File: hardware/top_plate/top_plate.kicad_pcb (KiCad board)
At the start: 2 copper layers, 96 x 66 mm, 36 parts, among them J1 Conn_01x04_Male, J2 Conn_01x04, J3 Conn_02x04_Odd_Even, J4 Conn_01x04, Q1 BSS138, Q2 BSS138, SW1 SW_Push, SW2 SW_Push, U1 AP2112K-1.8, U2 ICM-20948

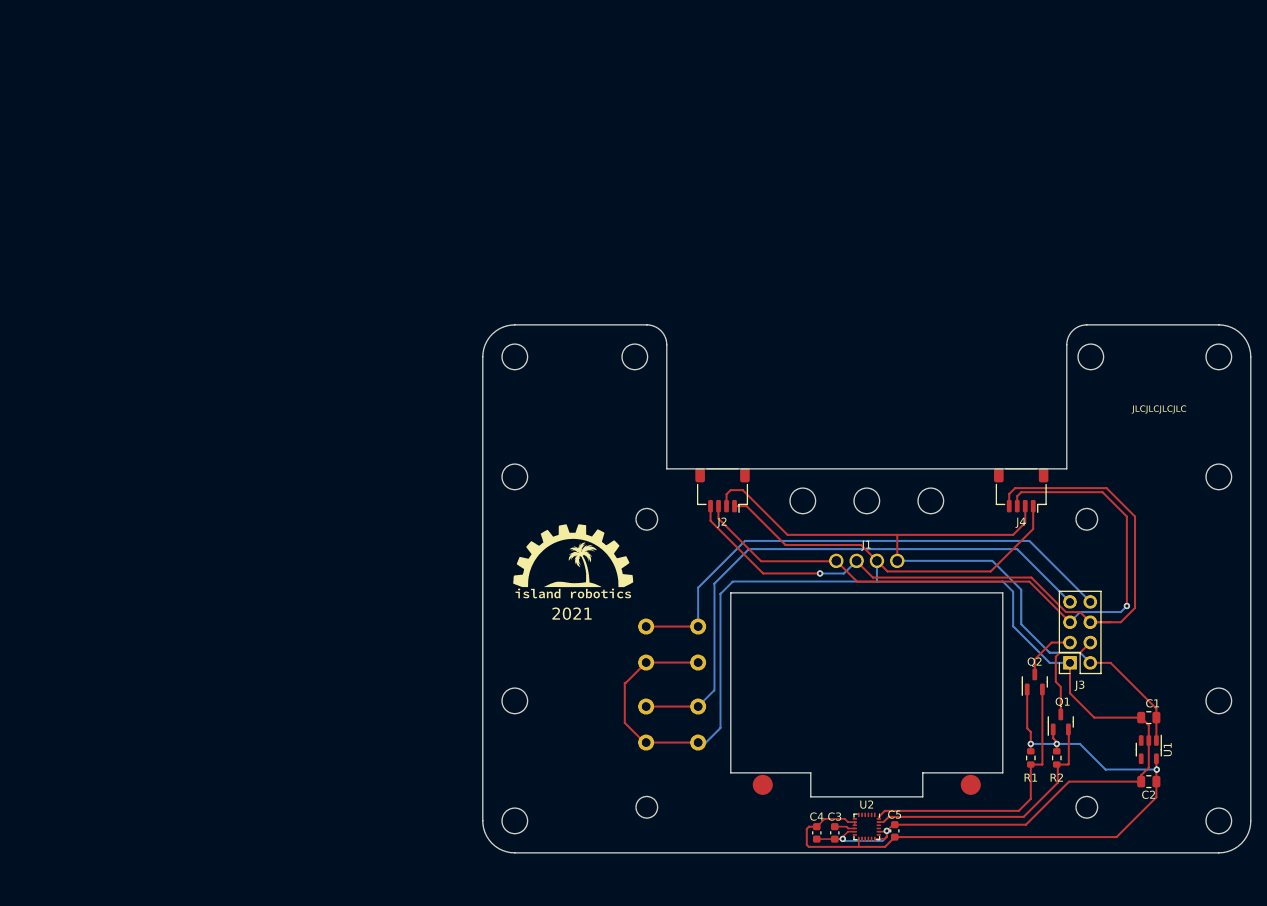
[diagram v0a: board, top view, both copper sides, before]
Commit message: Creating v4 branch
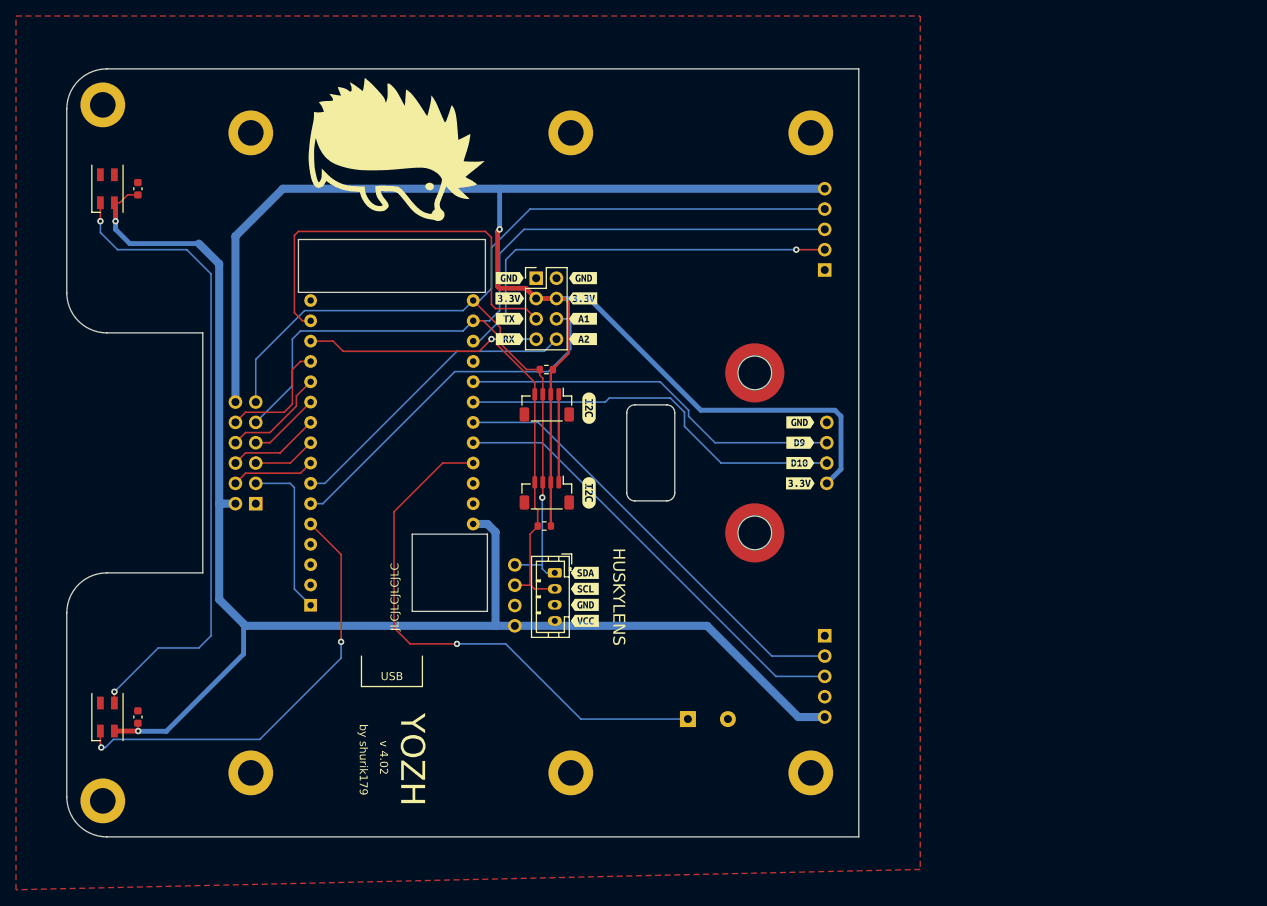
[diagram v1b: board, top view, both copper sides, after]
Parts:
- removed C3, C4, C5: 100nF, Capacitor_SMD:C_0603_1608Metric
- removed the G*** at (113.3, 113.5)
- removed J4: Conn_01x04, Connector_JST:JST_SH_SM04B-SRSS-TB_1x04-1MP_P1.00mm_Horizontal
- removed Q1, Q2: BSS138, Package_TO_SOT_SMD:SOT-23
- removed the REF** at (194.0, 131.0)
- removed the REF** at (150.0, 106.0)
- removed the REF** at (106.0, 146.0)
- removed the REF** at (122.5, 144.3)
- removed the REF** at (121.0, 88.0)
- removed the REF** at (158.0, 106.0)
- removed the REF** at (194.0, 146.0)
- removed the REF** at (194.0, 88.0)
- removed the REF** at (106.0, 131.0)
- removed the REF** at (177.5, 108.3)
- removed the REF** at (177.5, 144.3)
- removed the REF** at (194.0, 103.0)
- removed the REF** at (122.5, 108.3)
- removed the REF** at (142.0, 106.0)
- removed the REF** at (106.0, 88.0)
- removed the REF** at (106.0, 103.0)
- removed the REF** at (178.0, 88.0)
- removed SW1, SW2: SW_Push, Button_Switch_THT:SW_PUSH_6mm_H4.3mm
- removed U1: AP2112K-1.8, Package_TO_SOT_SMD:SOT-23-5
- removed U2: ICM-20948, Sensor_Motion:InvenSense_QFN-24_3x3mm_P0.4mm
- added A1: Adafruit_Feather_Generic, Module:Adafruit_Feather, B.Cu at (80.5, 119.0)
- added BZ1: Buzzer, Buzzer_Beeper:Buzzer_TDK_PS1240P02BT_D12.2mm_H6.5mm, B.Cu at (127.6, 133.3)
- added D1: SK6812MINI, LED_SMD:LED_SK6812MINI_PLCC4_3.5x3.5mm_P1.75mm, F.Cu at (55.1, 133.0)
- added D2: SK6812MINI, LED_SMD:LED_SK6812MINI_PLCC4_3.5x3.5mm_P1.75mm, F.Cu at (55.1, 67.0)
- added J10: Conn_02x04_Odd_Even, Connector_PinHeader_2.54mm:PinHeader_2x04_P2.54mm_Vertical, F.Cu at (108.7, 78.2)
- added J5: Conn_01x04, Connector_JST:JST_PH_B4B-PH-K_1x04_P2.00mm_Vertical, F.Cu at (111.0, 115.0)
- added J6: Conn_01x04, shurik-personal:connector-4p-generic-nosilk, F.Cu at (145.0, 103.8)
- added J7: Conn_01x04, shurik-personal:connector-4p-generic-nosilk, F.Cu at (106.0, 114.0)
- added J8: Conn_01x04, Connector_JST:JST_SH_BM04B-SRSS-TB_1x04-1MP_P1.00mm_Vertical, F.Cu at (110.0, 105.0)
- added J9: Conn_01x04, Connector_JST:JST_SH_BM04B-SRSS-TB_1x04-1MP_P1.00mm_Vertical, F.Cu at (110.0, 94.0)
- added M1: SMTSO3035, shurik-personal:mounting_SMD_NUT_M3_H6mm, F.Cu at (136.0, 90.0)
- added M2: SMTSO3035, shurik-personal:mounting_SMD_NUT_M3_H6mm, F.Cu at (136.0, 110.0)
- added REF**: MountingHole_3.2mm_M3_DIN965_Pad, MountingHole:MountingHole_3.2mm_M3_DIN965_Pad, F.Cu at (54.5, 143.5)
- added REF**: MountingHole_3.2mm_M3_DIN965_Pad, MountingHole:MountingHole_3.2mm_M3_DIN965_Pad, F.Cu at (113.0, 140.0)
- added REF**: MountingHole_3.2mm_M3_DIN965_Pad, MountingHole:MountingHole_3.2mm_M3_DIN965_Pad, F.Cu at (54.5, 56.5)
- added REF**: MountingHole_3.2mm_M3_DIN965_Pad, MountingHole:MountingHole_3.2mm_M3_DIN965_Pad, F.Cu at (143.0, 60.0)
- added REF**: MountingHole_3.2mm_M3_DIN965_Pad, MountingHole:MountingHole_3.2mm_M3_DIN965_Pad, F.Cu at (113.0, 60.0)
- added REF**: MountingHole_3.2mm_M3_DIN965_Pad, MountingHole:MountingHole_3.2mm_M3_DIN965_Pad, F.Cu at (143.0, 140.0)
- added REF**: MountingHole_3.2mm_M3_DIN965_Pad, MountingHole:MountingHole_3.2mm_M3_DIN965_Pad, F.Cu at (73.0, 140.0)
- added REF**: MountingHole_3.2mm_M3_DIN965_Pad, MountingHole:MountingHole_3.2mm_M3_DIN965_Pad, F.Cu at (73.0, 60.0)
- added kibuzzard-653BCB65: G***, kibuzzard-653BCB65, F.Cu at (115.3, 105.0)
- added kibuzzard-653BCB65: G***, kibuzzard-653BCB65, F.Cu at (115.3, 94.4)
- added kibuzzard-653BCCF1: G***, kibuzzard-653BCCF1, F.Cu at (114.8, 119.0)
- added kibuzzard-653BCCF1: G***, kibuzzard-653BCCF1, F.Cu at (114.5, 78.2)
- added kibuzzard-653BCD2B: G***, kibuzzard-653BCD2B, F.Cu at (114.5, 80.7)
- added kibuzzard-653BCD42: G***, kibuzzard-653BCD42, F.Cu at (114.5, 83.2)
- added kibuzzard-653BCD4B: G***, kibuzzard-653BCD4B, F.Cu at (114.5, 85.8)
- added kibuzzard-653BCDC1: G***, kibuzzard-653BCDC1, F.Cu at (141.7, 96.2)
- added kibuzzard-653BCDC1: G***, kibuzzard-653BCDC1, F.Cu at (105.4, 78.2)
- added kibuzzard-653BCDD4: G***, kibuzzard-653BCDD4, F.Cu at (105.4, 80.7)
- added kibuzzard-653BCDDF: G***, kibuzzard-653BCDDF, F.Cu at (105.4, 83.2)
- added kibuzzard-653BCDE7: G***, kibuzzard-653BCDE7, F.Cu at (105.4, 85.8)
- added kibuzzard-653BCECF: G***, kibuzzard-653BCECF, F.Cu at (114.8, 115.0)
- added kibuzzard-653BCED5: G***, kibuzzard-653BCED5, F.Cu at (114.8, 117.0)
- added kibuzzard-653BCEE0: G***, kibuzzard-653BCEE0, F.Cu at (114.8, 121.0)
- added kibuzzard-653BCF3B: G***, kibuzzard-653BCF3B, F.Cu at (141.7, 103.8)
- added kibuzzard-653BCF42: G***, kibuzzard-653BCF42, F.Cu at (141.7, 101.3)
- added kibuzzard-653BCF4B: G***, kibuzzard-653BCF4B, F.Cu at (141.7, 98.7)
- C1, C2: value 1uF -> 100nF; footprint Capacitor_SMD:C_0805_2012Metric -> Capacitor_SMD:C_0603_1608Metric
- G***: moved to F.Cu
- J1: value Conn_01x04_Male -> Conn_01x05; footprint shurik-personal:OLED_128x64_1_3in -> Connector_PinHeader_2.54mm:PinHeader_1x05_P2.54mm_Horizontal; moved to B.Cu
- J2: value Conn_01x04 -> Conn_02x06_Odd_Even; footprint Connector_JST:JST_SH_SM04B-SRSS-TB_1x04-1MP_P1.00mm_Horizontal -> Connector_PinSocket_2.54mm:PinSocket_2x06_P2.54mm_Vertical; moved to B.Cu
- J3: value Conn_02x04_Odd_Even -> Conn_01x05; footprint Connector_PinSocket_2.54mm:PinSocket_2x04_P2.54mm_Vertical -> Connector_PinHeader_2.54mm:PinHeader_1x05_P2.54mm_Horizontal; moved to B.Cu
- R1, R2: value 10K -> 3.3K
- moved C2 146.5 mm to (58.9, 67.0), turned to 90 degrees
- moved C1 126.4 mm to (58.9, 133.0), turned to 90 degrees
- moved G*** 103.3 mm to (91.1, 61.1), turned to -90 degrees
- moved R2 80.2 mm to (109.9, 89.6), turned to 180 degrees
- moved R1 67.4 mm to (109.7, 109.1), turned to 180 degrees
- moved J2 58.4 mm to (73.6, 106.3), turned to 0 degrees
- moved J3 57.9 mm to (144.7, 77.1), turned to 0 degrees
- moved J1 12.1 mm to (144.7, 122.9), turned to 180 degrees
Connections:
- C1 pad 1: +3V3 -> VCC
- C1 pad 2: GNDREF -> GND
- C2 pad 1: +1V8 -> VCC
- C2 pad 2: GNDREF -> GND
- J1 pad 1: +3V3 -> GND
- J1 pad 2: GNDREF -> /D11-XSHUT2
- J1 pad 3: /SCL -> /D12
- J1 pad 4: /SDA -> unconnected-(J1-Pin_4-Pad4)
- J2 pad 1: GNDREF -> GND
- J2 pad 2: +3V3 -> VCC
- J2 pad 3: /SDA -> /RESET
- J2 pad 4: /SCL -> /A3
- J3 pad 1: GNDREF -> GND
- J3 pad 2: +3V3 -> /D5-XSHUT1
- J3 pad 3: /SDA1 -> /SCL
- J3 pad 4: /SCL1 -> /SDA
- J3 pad 5: /SDA -> +3V3
- R1 pad 1: +1V8 -> +3V3
- R1 pad 2: /SDA_1V8 -> /SCL
- R2 pad 1: +1V8 -> +3V3
- R2 pad 2: /SCL_1V8 -> /SDA
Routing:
- net GNDREF: track 217.2 -> 0.00 mm, vias 2 -> 0
- net VCC: track 0.00 -> 187.8 mm, vias 0 -> 2
- net +3V3: track 93.9 -> 198.2 mm, vias 0 -> 1
- net +1V8: track 89.2 -> 0.00 mm, vias 3 -> 0
- net Net-(D1-DOUT): track 0.00 -> 81.3 mm, vias 0 -> 2
- net /B: track 71.7 -> 0.00 mm
- net /D13-BUZZ: track 0.00 -> 68.4 mm, vias 0 -> 1
- net /A: track 66.0 -> 0.00 mm
- net /D11-XSHUT2: track 0.00 -> 56.0 mm
- net /D12: track 0.00 -> 56.0 mm
- net /NEOPXL: track 0.00 -> 55.1 mm, vias 0 -> 2
- net /D5-XSHUT1: track 0.00 -> 52.7 mm, vias 0 -> 1
- net /TX: track 0.00 -> 52.0 mm
- net /D10: track 0.00 -> 48.8 mm
- net /D9: track 0.00 -> 47.8 mm
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- added copper zone on F.Cu, net GND
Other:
- board size 96 x 66 mm -> 99 x 96 mm
- board text added: "HUSKYLENS"
- board text added: "USB"
- board text added: "YOZH"
- board text added: "by shurik179"
- board text added: "v 4.02"
- board text removed: "2021"
- board text removed: "A"
- board text removed: "B"
- board text removed: "Yozh Robot v2.0"
- board text removed: "yozh.rtfd.io"
